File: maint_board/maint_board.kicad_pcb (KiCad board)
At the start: 2 copper layers, 133.3 x 97.2 mm, 88 parts, among them J2 4P4C, K1 KEYSW, K10 KEYSW, K11 KEYSW, K12 KEYSW, K13 KEYSW, K15 KEYSW, K16 KEYSW, K17 KEYSW, K18 KEYSW, K19 KEYSW, K2 KEYSW, K20 KEYSW, K29 KEYSW, K3 KEYSW, K30 KEYSW, K31 KEYSW, K4 KEYSW, K5 KEYSW, K6 KEYSW, K8 KEYSW, K9 KEYSW, Q1 Q_NMOS_GSD, SW1 SW_PUSH, U1 ATMEGA32U4, X1 XTAL_GND

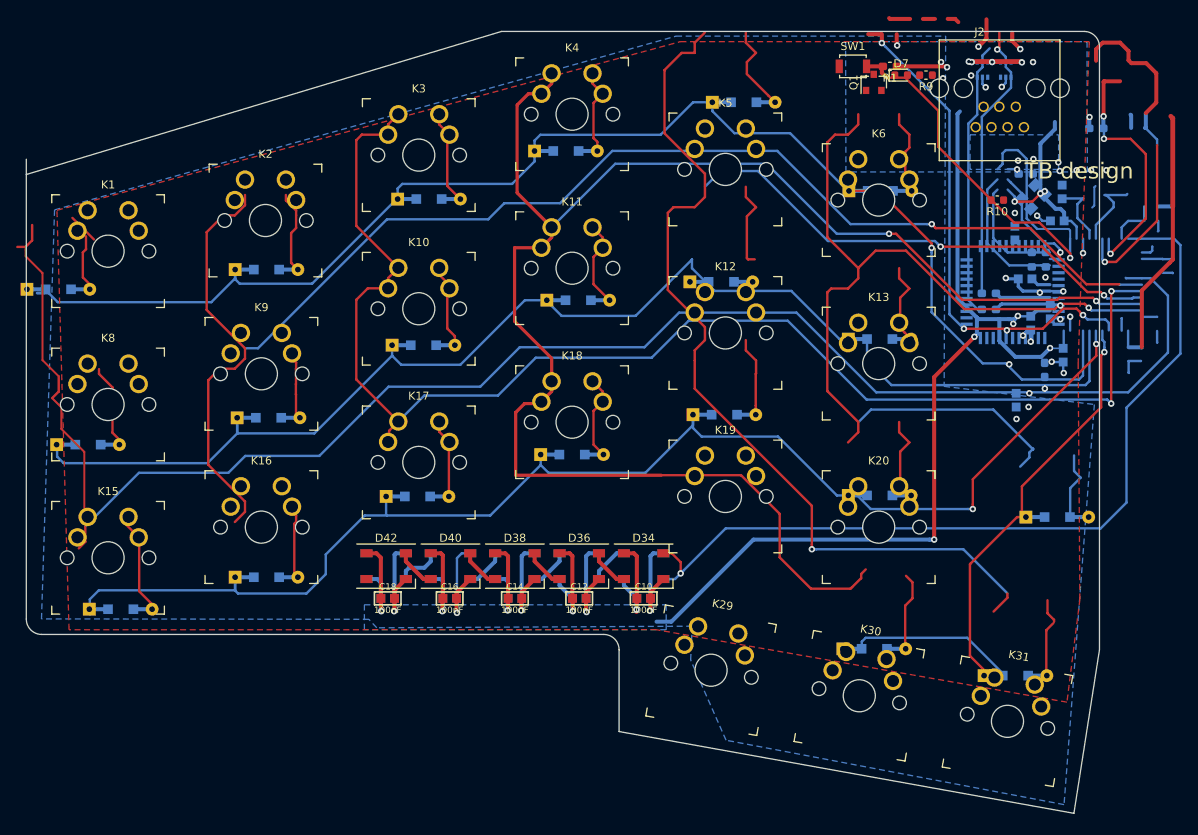
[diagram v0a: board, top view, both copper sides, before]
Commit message: this is before I switch to usb C
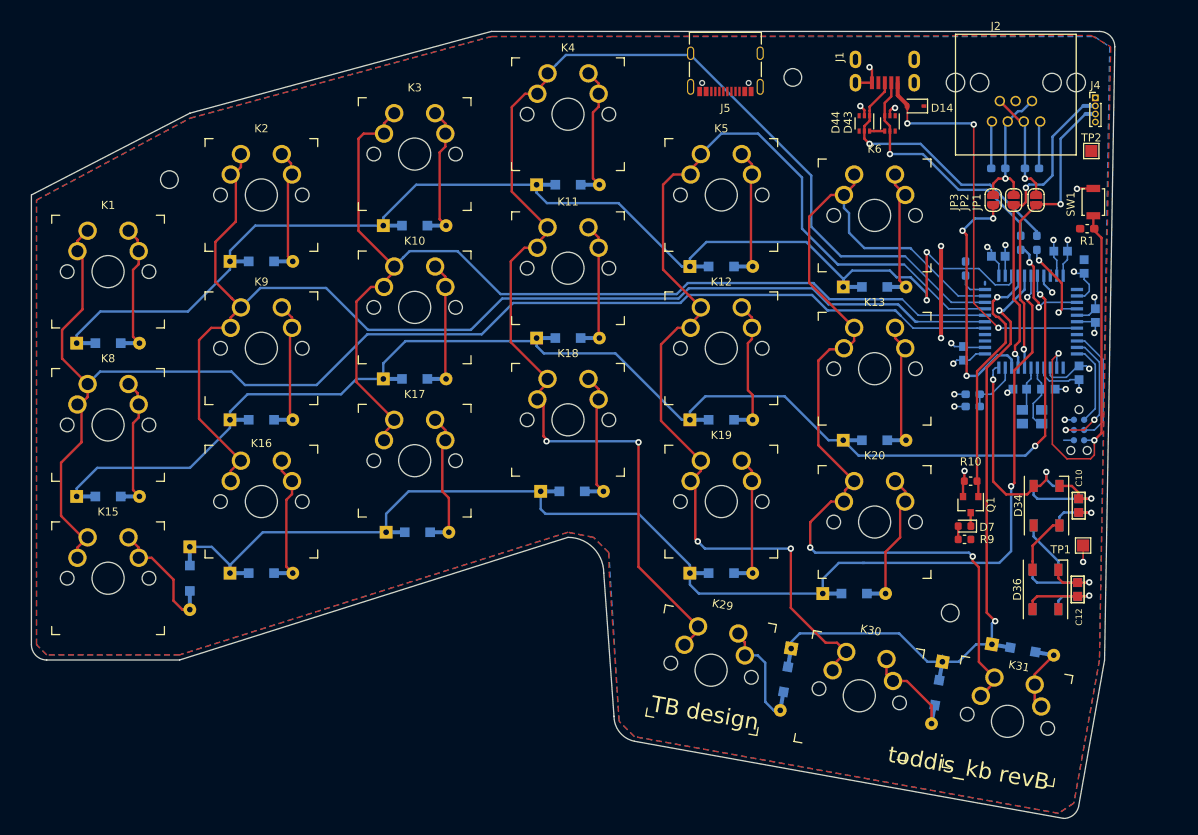
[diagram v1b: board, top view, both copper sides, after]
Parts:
- removed C13, C14, C15, C16, C17, C18: 100nF, keyboard_parts:C_1608
- removed D37, D38, D39, D40, D41, D42: SK6812, LED_SMD:LED_SK6812_PLCC4_5.0x5.0mm_P3.2mm
- added D14: 1N4148W, Diode_SMD:D_SOD-323, F.Cu at (170.2, 42.9)
- added H1: MountingHole, MountingHole:MountingHole_2.2mm_M2_ISO7380, F.Cu at (77.5, 52.1)
- added H2: MountingHole, MountingHole:MountingHole_2.2mm_M2_ISO7380, F.Cu at (154.9, 39.4)
- added H3: MountingHole, MountingHole:MountingHole_2.2mm_M2_ISO7380, F.Cu at (174.5, 105.9)
- added J1: USB_mini_micro_B, TB_connectors:usb_minib_wm5462ct-nd, F.Cu at (166.4, 36.8)
- added J3: TC2030-IDC_FB, Connector:Tag-Connect_TC2030-IDC-NL_2x03_P1.27mm_Vertical, B.Cu at (190.5, 83.2)
- added J4: Conn_01x04, Connector_PinHeader_1.00mm:PinHeader_1x04_P1.00mm_Vertical, F.Cu at (192.5, 41.9)
- added J5: USB_C_Receptacle_USB2.0, Connector_USB:USB_C_Receptacle_Palconn_UTC16-G, F.Cu at (146.6, 38.6)
- added JP1: SolderJumper_2_Open, Jumper:SolderJumper-2_P1.3mm_Open_RoundedPad1.0x1.5mm, F.Cu at (185.2, 54.6)
- added JP2: SolderJumper_2_Open, Jumper:SolderJumper-2_P1.3mm_Open_RoundedPad1.0x1.5mm, F.Cu at (182.4, 54.6)
- added JP3: SolderJumper_2_Open, Jumper:SolderJumper-2_P1.3mm_Open_RoundedPad1.0x1.5mm, F.Cu at (179.8, 54.6)
- added TP1: TestPoint_Flag, TestPoint:TestPoint_Pad_1.5x1.5mm, F.Cu at (191.0, 97.5)
- added TP2: TestPoint_Flag, TestPoint:TestPoint_Pad_1.5x1.5mm, F.Cu at (192.0, 48.5)
- D43, D44: moved to F.Cu
- J2: footprint my_connectors:glx-n-44_reverseble -> TB_connectors:glx-n-44_reverseble
- moved C11 61.9 mm to (190.3, 103.0), turned to 90 degrees
- moved C12 61.9 mm to (190.3, 103.0), turned to 90 degrees
- moved D35 58.0 mm to (186.3, 103.0), turned to 90 degrees
- moved D36 58.0 mm to (186.3, 103.0), turned to 90 degrees
- moved R9 57.9 mm to (176.3, 96.8)
- moved D7 56.6 mm to (176.3, 95.1), turned to 180 degrees
- moved C10 55.3 mm to (190.5, 92.6), turned to 90 degrees
- moved C9 55.3 mm to (190.5, 92.6), turned to 90 degrees
- moved Q1 53.8 mm to (177.0, 92.5), turned to 270 degrees
- moved D33 50.6 mm to (186.5, 92.6), turned to 90 degrees
- moved D34 50.6 mm to (186.5, 92.6), turned to 90 degrees
- moved R10 35.1 mm to (177.0, 89.5)
- moved SW1 34.3 mm to (192.3, 54.9), turned to 270 degrees
- moved R1 31.7 mm to (191.5, 58.2), turned to 0 degrees
- moved X1 27.3 mm to (184.7, 81.5), turned to 180 degrees
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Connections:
- U1 pad 18: /mcu/SCL -> i2c_scl
- U1 pad 19: /mcu/SDA -> i2c_sda
- U1 pad 20: Net-(U1-Pad20) -> serial
- U1 pad 36: Net-(U1-Pad36) -> /keys/Row1
- U1 pad 41: /keys/Row1 -> Net-(U1-Pad41)
- U1 pad 7: Net-(U1-Pad7) -> /mcu/Vbus
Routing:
- net VCC: track 273.2 -> 61.8 mm, vias 23 -> 9
- net /keys/Col5: track 262.1 -> 139.8 mm, vias 5 -> 2
- net /keys/Col6: track 27.4 -> 124.9 mm, vias 1 -> 2
- net /Leds/Din: track 107.1 -> 26.7 mm, vias 1 -> 2
- net (no net): track 50.8 -> 0.35 mm
- net /mcu/Vbus: track 0.00 -> 50.2 mm, vias 0 -> 3
- net /keys/Col1: track 210.2 -> 167.2 mm, vias 1 -> 0
- net i2c_sda: track 0.00 -> 40.0 mm, vias 0 -> 2
- net /keys/Col3: track 169.1 -> 129.8 mm, vias 2 -> 0
- net i2c_scl: track 0.00 -> 38.1 mm, vias 0 -> 2
- net /keys/Col4: track 201.0 -> 168.2 mm
- net serial: track 0.00 -> 32.2 mm, vias 0 -> 3
- net Net-(Q1-Pad1): track 63.1 -> 31.8 mm, vias 3 -> 1
- net /keys/Row1: track 177.8 -> 148.4 mm, vias 1 -> 2
- net /mcu/SCL: track 42.6 -> 14.2 mm, vias 3 -> 1
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- added copper zone on F.Cu, net VCC
- removed copper zone on F.Cu, net GND
- removed copper zone on B.Cu, net VCC
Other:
- board size 133.3 x 97.2 mm -> 134.6 x 97.8 mm
- net class Min: clearance 0.1 -> 0.2; trace_width 0.1 -> 0.2
- rule trace_min: 0.1 -> 0.2
- board text added: "toddis_kb revB"
